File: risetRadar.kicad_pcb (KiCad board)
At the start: 2 copper layers, 60.3 x 50.4 mm, 122 parts, among them Q1 MBT3904DW1, U1 XC7A35T-FTG256, U2 LTC3569EUDC, U3 MT41J128M16JT-125:KTR, U4 FT2232HL, U5 MT25QL128ABA1ESE-MSITTR, U6 93LC46BT-I/OT, Y1 Crystal_GND24

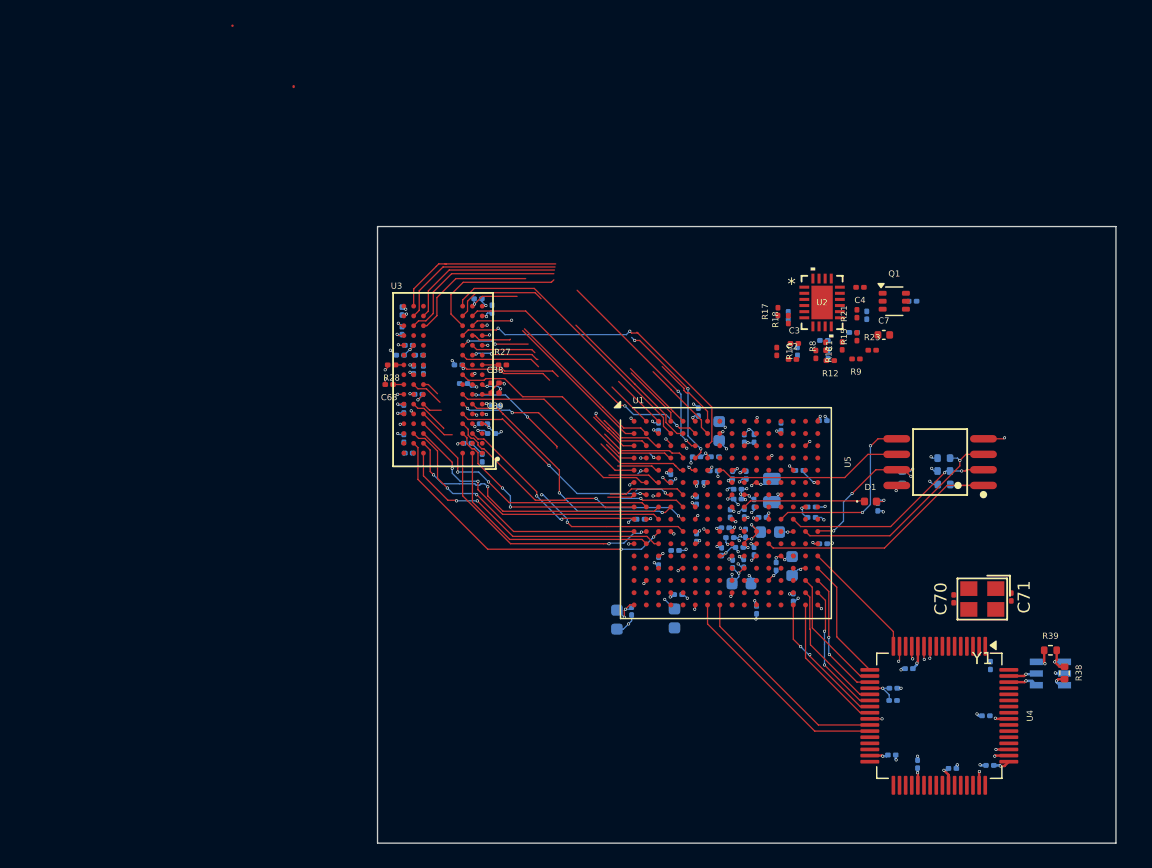
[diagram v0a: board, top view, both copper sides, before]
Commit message: add
add
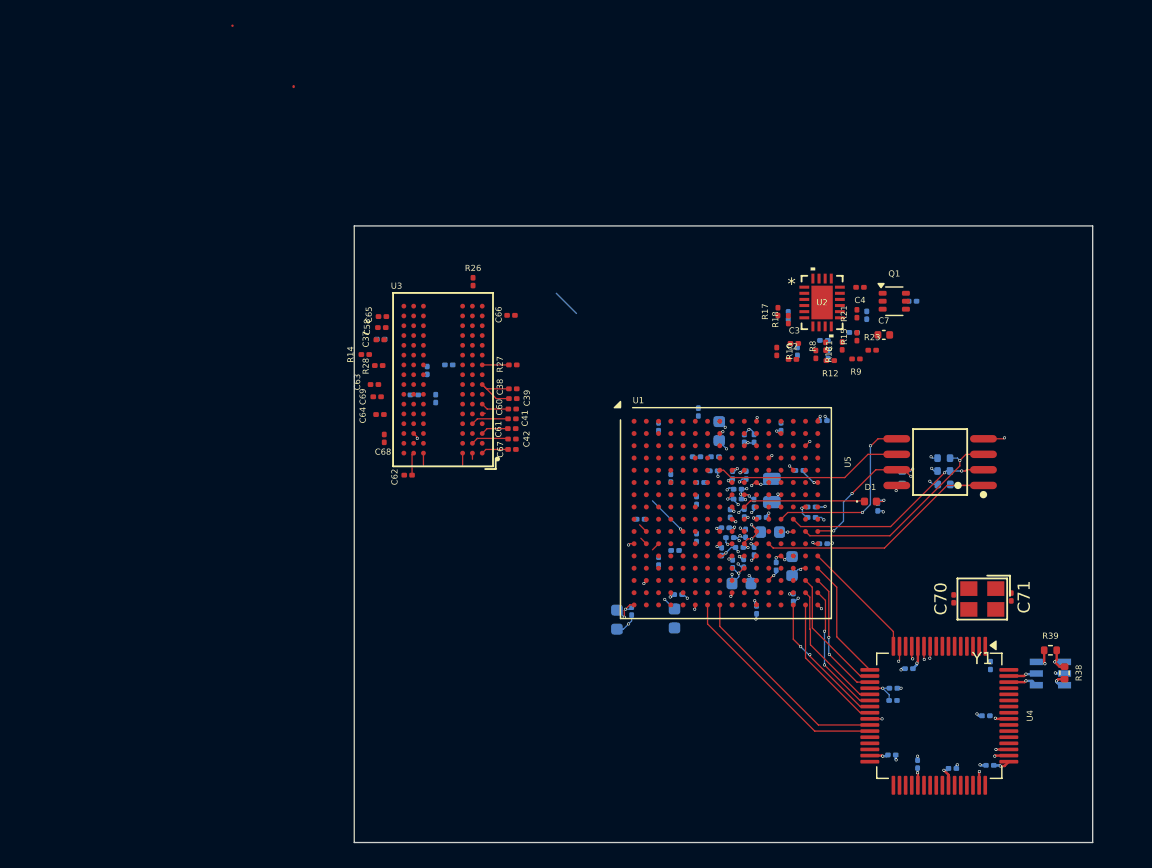
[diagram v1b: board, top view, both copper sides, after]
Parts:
- C37, C41, C42, C58, C60, C61, C62, C64, C65, C66, C67, C68, C69, R14, R26: moved to F.Cu
- moved R14 4.40 mm to (90.9, 71.6), turned to 180 degrees
- moved C69 3.70 mm to (91.9, 75.0), turned to 180 degrees
- moved C42 3.65 mm to (102.9, 78.5), turned to 0 degrees
- moved C59 2.59 mm to (96.7, 75.2), turned to -90 degrees
- moved C67 2.53 mm to (102.9, 79.3), turned to 0 degrees
- moved C41 2.36 mm to (102.9, 76.8)
- moved C40 2.33 mm to (92.2, 70.3)
- moved C37 2.05 mm to (92.1, 70.4)
- moved C64 2.00 mm to (92.1, 76.5), turned to 180 degrees
- moved C62 1.80 mm to (94.4, 81.5)
- moved C61 1.71 mm to (102.9, 77.7)
- moved C58 1.67 mm to (92.2, 69.4), turned to 180 degrees
- moved C65 1.66 mm to (92.3, 68.5), turned to 180 degrees
- moved C66 1.63 mm to (102.8, 68.4), turned to 0 degrees
- moved C68 1.60 mm to (92.5, 78.5)
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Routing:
- net /FPGA/FPGAIO2/DDR3_ADDR8: track 27.4 -> 0.00 mm
- net /FPGA/FPGAIO2/DDR3_ADDR0: track 26.9 -> 0.00 mm, vias 2 -> 0
- net /FPGA/FPGAIO2/DDR3_DQ14: track 25.7 -> 0.00 mm, vias 2 -> 0
- net GNDREF: track 68.2 -> 43.6 mm, vias 95 -> 56
- net /FPGA/FPGAIO2/DDR3_ADDR1: track 23.4 -> 0.00 mm
- net /FPGA/FPGAIO2/DDR3_DQS_1_N: track 23.2 -> 0.00 mm, vias 2 -> 0
- net /FPGA/FPGAIO2/DDR3_ADDR13: track 23.2 -> 0.00 mm
- net /FPGA/FPGAIO2/DDR3_DQS_1_P: track 23.0 -> 0.00 mm, vias 2 -> 0
- net /FPGA/FPGAIO2/DDR3_ADDR7: track 22.5 -> 0.00 mm, vias 2 -> 0
- net /FPGA/FPGAIO2/DDR3_DQ10: track 22.6 -> 0.52 mm, vias 2 -> 1
- net /FPGA/FPGAIO2/DDR3_DM_1: track 21.8 -> 0.00 mm, vias 2 -> 0
- net /FPGA/FPGAIO2/DDR3_DQ12: track 23.4 -> 1.76 mm, vias 2 -> 0
- net /FPGA/FPGAIO2/DDR3_DQ8: track 21.7 -> 0.00 mm, vias 2 -> 0
- net /FPGA/FPGAIO2/DDR3_DQ2: track 21.2 -> 0.00 mm, vias 2 -> 0
- net /FPGA/FPGAIO2/DDR3_ADDR9: track 20.7 -> 0.00 mm
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
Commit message: add
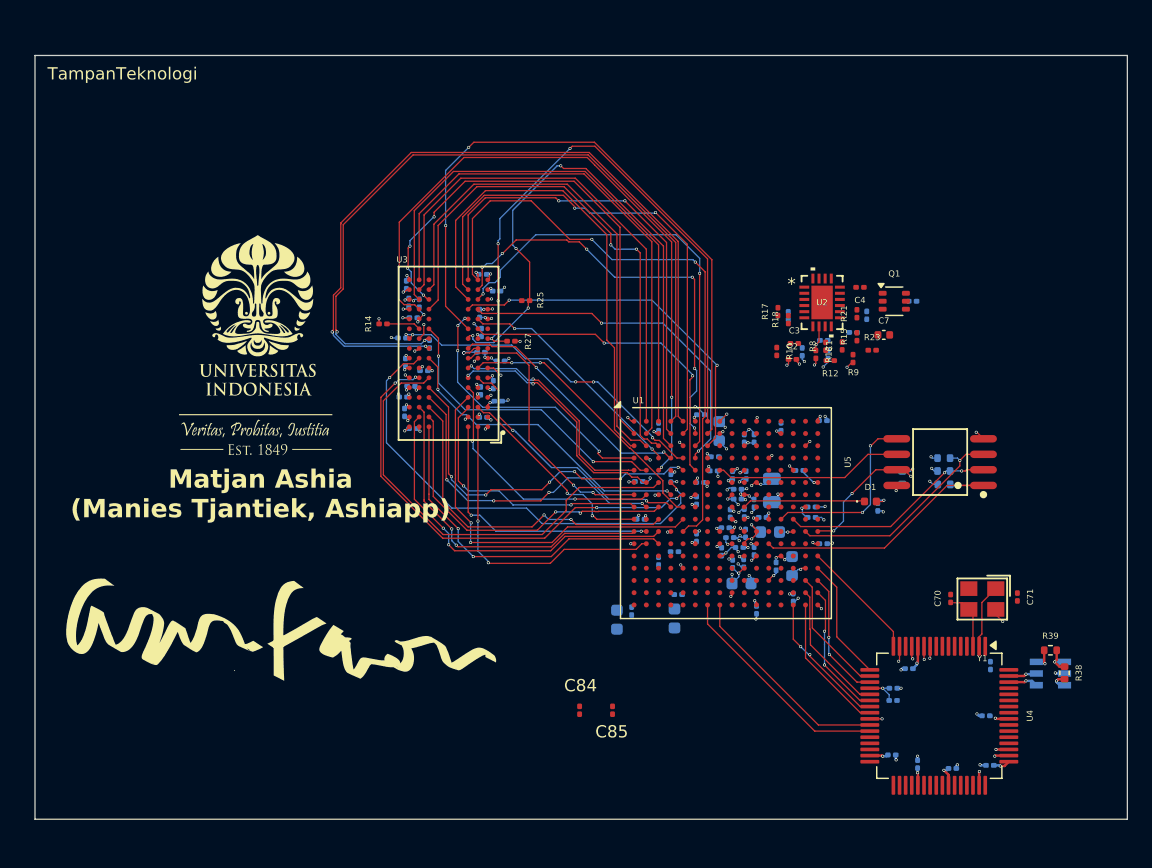
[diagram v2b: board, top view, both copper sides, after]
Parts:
- added C84: 0.47uF, Capacitor_SMD:C_0201_0603Metric, F.Cu at (108.4, 100.7)
- added C85: 0.47uF, Capacitor_SMD:C_0201_0603Metric, F.Cu at (111.1, 100.7)
- C37, C38, C39, C41, C42, C58, C60, C61, C62, C63, C64, C65, C66, C67, C68, C69, R26, R28: moved to B.Cu
- R25: moved to F.Cu
- moved C67 11.4 mm to (100.2, 68.2), turned to -90 degrees
- moved R25 8.19 mm to (104.0, 67.2)
- moved C59 6.57 mm to (100.4, 69.8), turned to 90 degrees
- moved C53 5.12 mm to (113.2, 82.0), turned to 0 degrees
- moved C39 4.60 mm to (100.3, 71.4), turned to 180 degrees
- moved C69 4.37 mm to (95.7, 72.9)
- moved C40 4.30 mm to (95.3, 67.4), turned to 90 degrees
- moved C62 3.82 mm to (94.8, 77.7)
- moved C64 3.43 mm to (94.6, 74.2), turned to 0 degrees
- moved C41 3.43 mm to (100.3, 74.6), turned to 90 degrees
- moved C42 3.29 mm to (101.8, 75.4)
- moved C65 3.25 mm to (94.2, 65.9), turned to 90 degrees
- moved C37 3.24 mm to (94.8, 68.6)
- moved C63 3.10 mm to (94.2, 72.2), turned to -90 degrees
- moved C58 3.01 mm to (94.5, 67.3), turned to 90 degrees
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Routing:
- net /FPGA/FPGAIO2/DDR3_CK_P: track 0.00 -> 65.9 mm, vias 0 -> 2
- net /FPGA/FPGAIO2/DDR3_CK_N: track 0.00 -> 65.0 mm, vias 0 -> 2
- net /FPGA/FPGAIO2/DDR3_WE_N: track 0.00 -> 54.7 mm, vias 0 -> 2
- net /FPGA/FPGAIO2/DDR3_BA1: track 0.00 -> 54.7 mm, vias 0 -> 2
- net /FPGA/FPGAIO2/DDR3_CAS_N: track 0.00 -> 48.3 mm, vias 0 -> 4
- net /FPGA/FPGAIO2/DDR3_ODT: track 2.18 -> 48.2 mm, vias 0 -> 4
- net /FPGA/FPGAIO2/DDR3_ADDR4: track 0.00 -> 45.6 mm
- net /FPGA/FPGAIO2/DDR3_RESET_N: track 5.87 -> 50.5 mm, vias 1 -> 3
- net /FPGA/FPGAIO2/DDR3_ADDR12: track 0.00 -> 44.5 mm, vias 0 -> 2
- net /FPGA/FPGAIO2/DDR3_ADDR1: track 0.00 -> 43.9 mm, vias 0 -> 4
- net /FPGA/FPGAIO2/DDR3_ADDR8: track 0.00 -> 43.9 mm
- net /FPGA/FPGAIO2/DDR3_ADDR9: track 0.00 -> 42.6 mm, vias 0 -> 2
- net /FPGA/FPGAIO2/DDR3_ADDR11: track 0.00 -> 42.3 mm
- net /FPGA/FPGAIO2/DDR3_ADDR6: track 0.00 -> 42.1 mm
- net /FPGA/FPGAIO2/DDR3_ADDR2: track 0.00 -> 40.0 mm
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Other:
- board size 60.3 x 50.4 mm -> 89.2 x 62.4 mm
- board text added: "Matjan Ashia (Manies Tjantiek, Ashiapp)"
- board text added: "TampanTeknologi"
